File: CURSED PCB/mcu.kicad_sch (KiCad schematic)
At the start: 1 part, among them U3 STM32H733VGT6

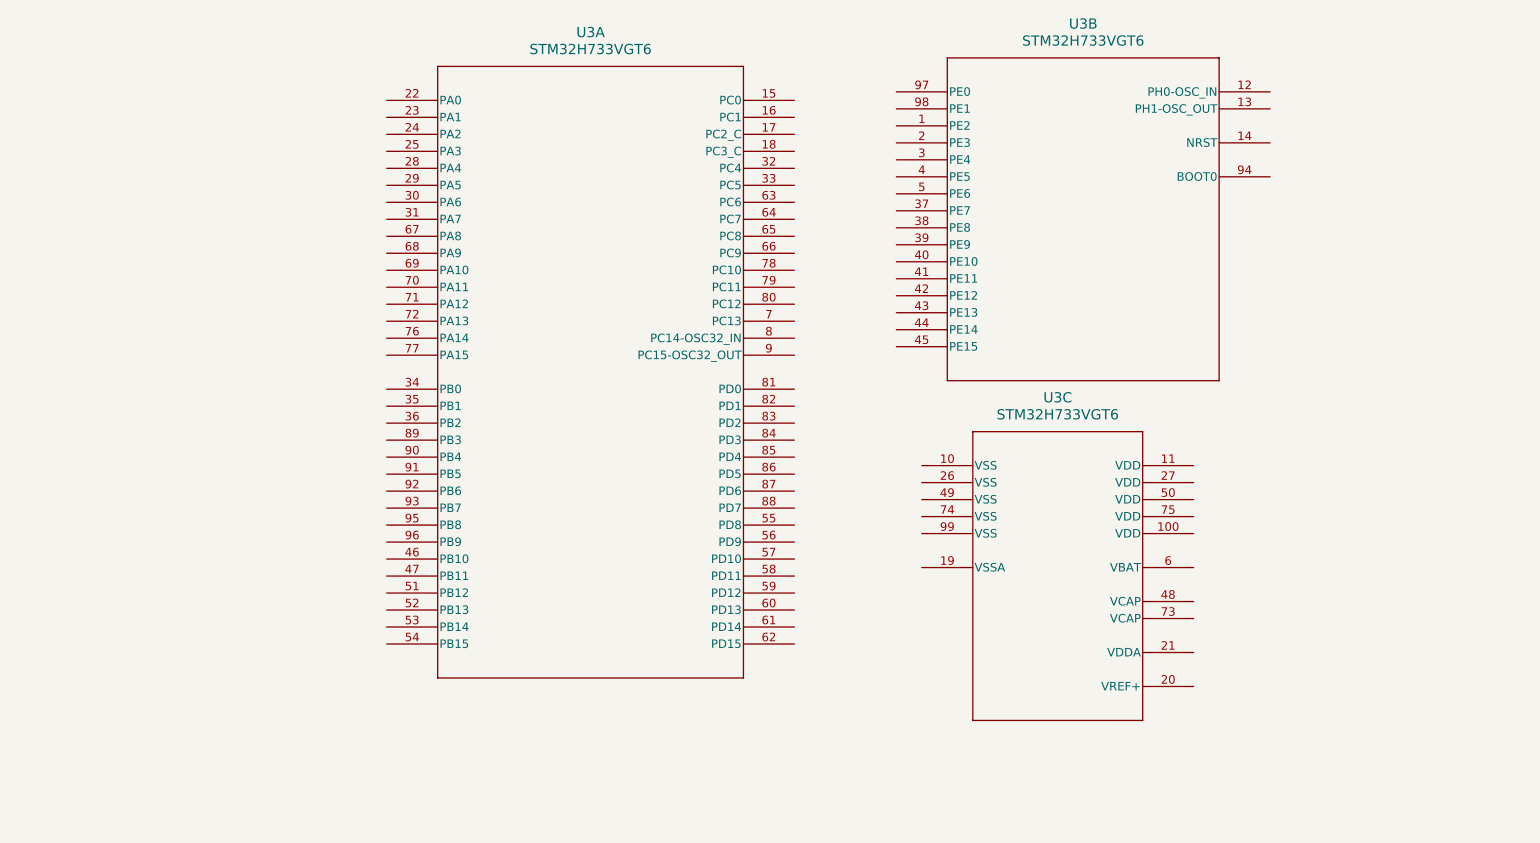
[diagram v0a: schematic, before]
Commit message: updated schematic
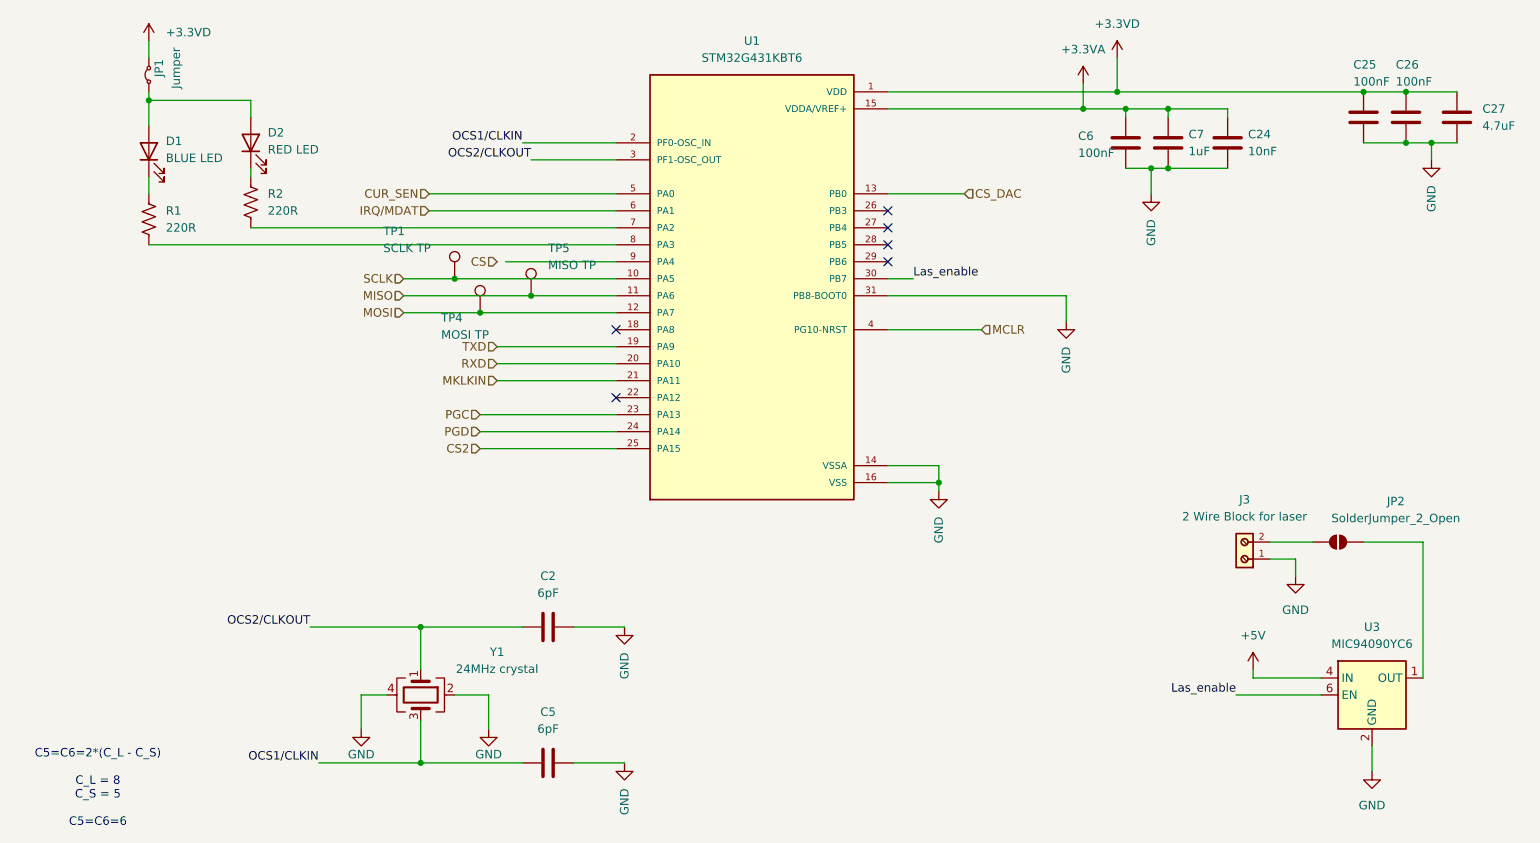
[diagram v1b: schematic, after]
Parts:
- removed U3: STM32H733VGT6, stm:LQFP100_STM, symbol STM32H733VGT6:STM32H733VGT6
- added C2, C5: 6pF, Capacitor_SMD:C_0805_2012Metric_Pad1.18x1.45mm_HandSolder, symbol PCM_Capacitor_US_AKL:C_0201
- added C24: 10nF, Capacitor_SMD:C_0805_2012Metric_Pad1.18x1.45mm_HandSolder, symbol PCM_Capacitor_US_AKL:C_0201
- added C25, C26, C6: 100nF, Capacitor_SMD:C_0805_2012Metric_Pad1.18x1.45mm_HandSolder, symbol PCM_Capacitor_US_AKL:C_0201
- added C27: 4.7uF, Capacitor_SMD:C_0805_2012Metric_Pad1.18x1.45mm_HandSolder, symbol PCM_Capacitor_US_AKL:C_0201
- added C7: 1uF, Capacitor_SMD:C_0805_2012Metric_Pad1.18x1.45mm_HandSolder, symbol PCM_Capacitor_US_AKL:C_0201
- added D1: BLUE LED, LED_SMD:LED_1206_3216Metric_Pad1.42x1.75mm_HandSolder, symbol Device:LED
- added D2: RED LED, LED_SMD:LED_1206_3216Metric_Pad1.42x1.75mm_HandSolder, symbol Device:LED
- added J3: 2 Wire Block for laser, 691137710002:691137710002, symbol 691137710002:691137710002
- added JP1: Jumper, Jumper:SolderJumper-2_P1.3mm_Bridged2Bar_Pad1.0x1.5mm, symbol Jumper:Jumper_2_Small_Bridged
- added JP2: SolderJumper_2_Open, Jumper:SolderJumper-2_P1.3mm_Open_Pad1.0x1.5mm, symbol Jumper:SolderJumper_2_Open
- added R1, R2: 220R, Resistor_SMD:R_0805_2012Metric_Pad1.20x1.40mm_HandSolder, symbol Device:R_US
- added TP1: SCLK TP, TestPoint:TestPoint_Pad_1.5x1.5mm, symbol Connector:TestPoint
- added TP4: MOSI TP, TestPoint:TestPoint_Pad_1.5x1.5mm, symbol Connector:TestPoint
- added TP5: MISO TP, TestPoint:TestPoint_Pad_1.5x1.5mm, symbol Connector:TestPoint
- added U1: STM32G431KBT6, STM32G431KBT6:QFP80P900X900X160-32N, symbol STM32G431KBT6:STM32G431KBT6
- added U3: MIC94090YC6, Package_TO_SOT_SMD:SOT-363_SC-70-6, symbol Power_Management:MIC94090YC6
- added Y1: 24MHz crystal, Crystal:Crystal_SMD_Abracon_ABM8G-4Pin_3.2x2.5mm, symbol Device:Crystal_GND24
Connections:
- new net: D2.1 (K), R2.1
- new net: D1.2 (A), D2.2 (A), JP1.1 (A)
- new net: R2.2, U1.7 (PA2)
- new net: R1.2, U1.8 (PA3)
- new net: D1.1 (K), R1.1
- new net: J3.2, JP2.1 (A)
- new net: JP2.2 (B), U3.1 (OUT)
- new net +3.3VA: C24.2, C6.1, C7.2, U1.15 (VDDA/VREF+)
- new net +3.3VD: C25.2, C26.2, C27.2, JP1.2 (B), U1.1 (VDD), U1.17 (VDD)
- new net +5V: U3.4 (IN)
- new net CS2: U1.25 (PA15)
- new net CS_DAC: U1.13 (PB0)
- new net CUR_SEN: U1.5 (PA0)
- new net GND: C2.2, C24.1, C25.1, C26.1, C27.1, C5.2, C6.2, C7.1, J3.1, U1.14 (VSSA), U1.16 (VSS), U1.31 (PB8-BOOT0), U1.32 (VSS), U3.2 (GND), U3.5 (GND), Y1.2, Y1.4
- new net IRQ/MDAT: U1.6 (PA1)
- new net Las_enable: U1.30 (PB7), U3.6 (EN)
- new net MCLR: U1.4 (PG10-NRST)
- new net MISO: TP5.1, U1.11 (PA6)
- new net MKLKIN: U1.21 (PA11)
- new net MOSI: TP4.1, U1.12 (PA7)
- new net OCS1/CLKIN: C5.1, U1.2 (PF0-OSC_IN), Y1.3
- new net OCS2/CLKOUT: C2.1, U1.3 (PF1-OSC_OUT), Y1.1
- new net PGC: U1.23 (PA13)
- new net PGD: U1.24 (PA14)
- new net RXD: U1.20 (PA10)
- new net SCLK: TP1.1, U1.10 (PA5)
- new net TXD: U1.19 (PA9)
- no-connect marks 0 -> 6
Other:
- note added: "C5=C6=2*(C_L - C_S) C_L = 8 C_S = 5 C5=C6=6"
